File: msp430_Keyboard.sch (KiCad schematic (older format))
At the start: 16 parts, among them J1 Conn_01x04_Male, SW14 L_Super, SW4 L_Ctrl, SW48 R_Ctrl, SW5 L_Shift, SW53 R_Shift, SW57 Alt_GR, SW60 R_Super, SW61 FUNC, SW9 L_Alt, U1 MSP430F5510IRGZ, Y1 12MHz, Y2 32.768kHz

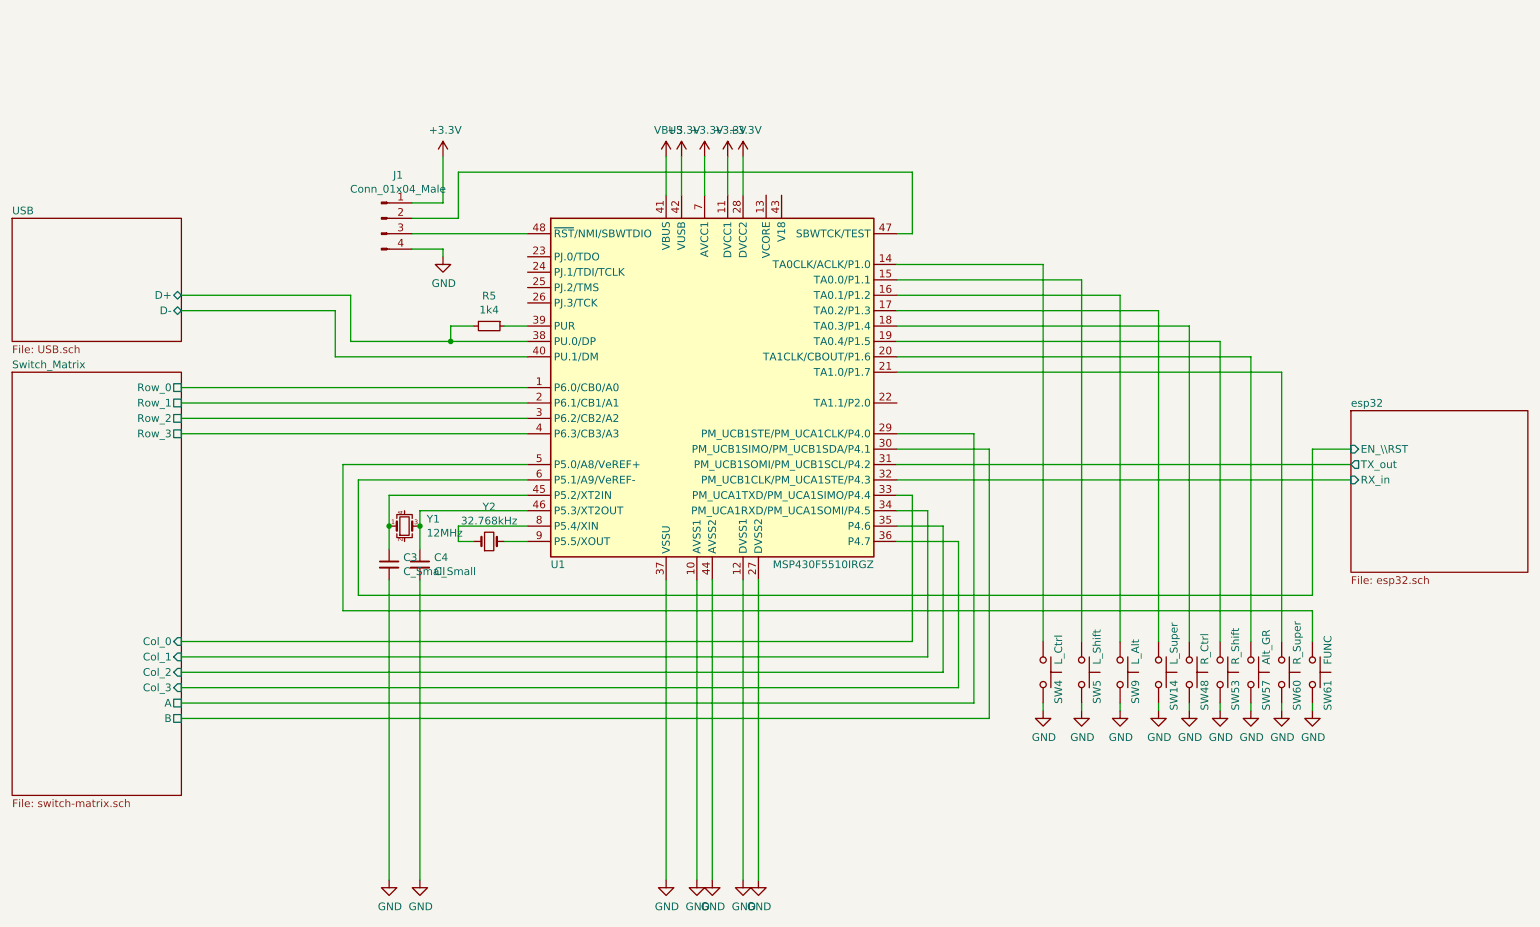
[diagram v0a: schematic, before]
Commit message: Routing angefangen
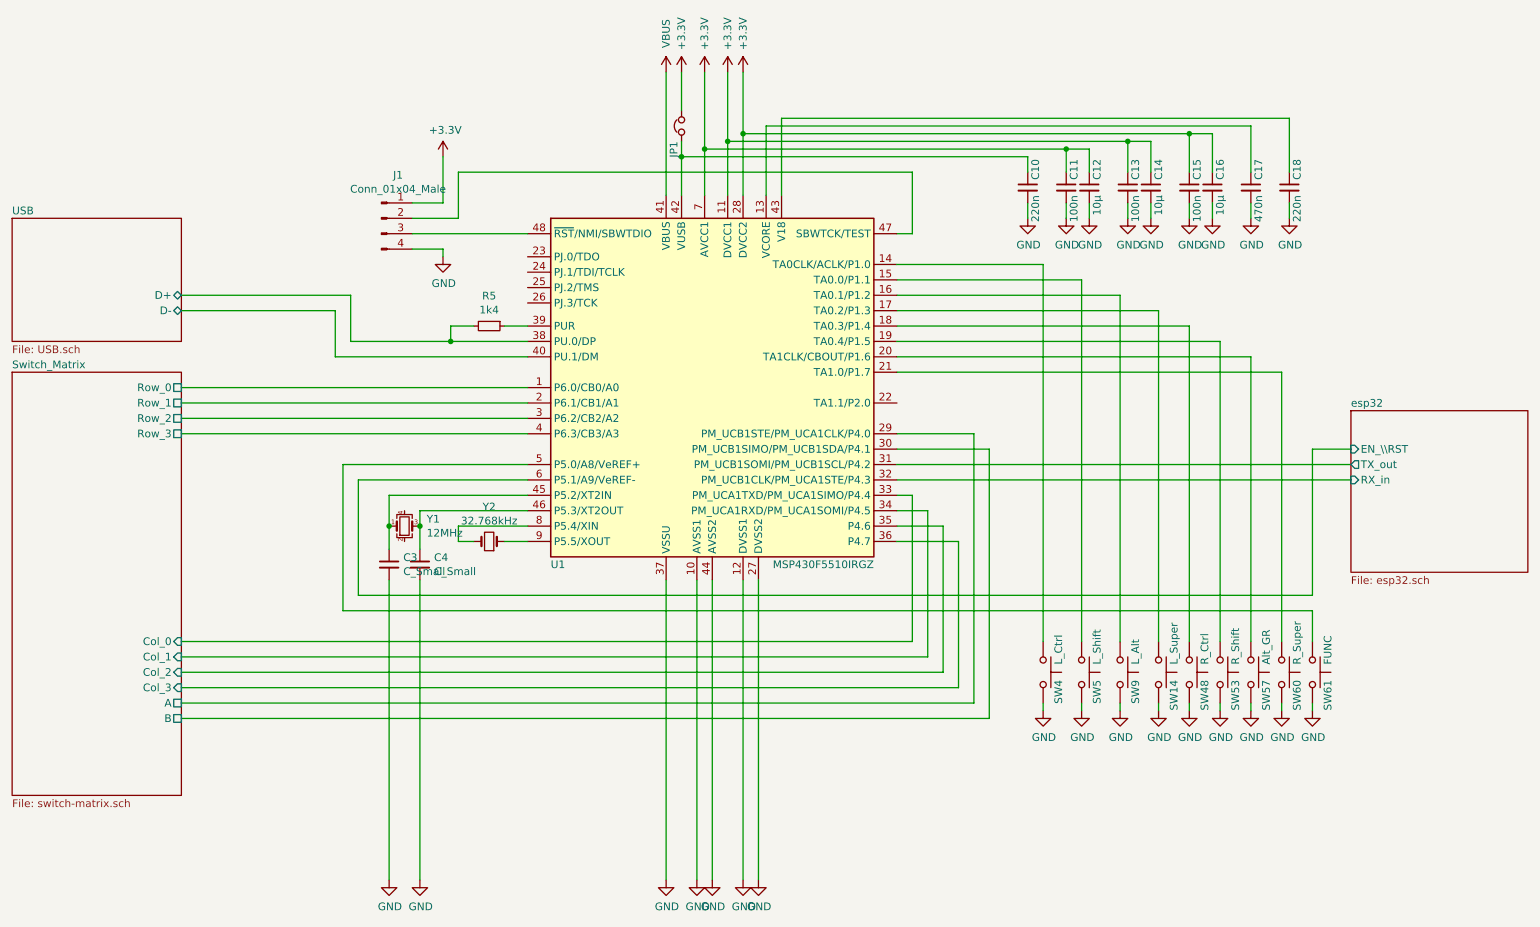
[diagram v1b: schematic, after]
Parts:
- added C10, C18: 220n, Capacitor_SMD:C_0603_1608Metric_Pad1.08x0.95mm_HandSolder, symbol Device:C_Small
- added C11, C13, C15: 100n, Capacitor_SMD:C_0603_1608Metric_Pad1.08x0.95mm_HandSolder, symbol Device:C_Small
- added C12, C14, C16: 10µ, Capacitor_SMD:C_1206_3216Metric_Pad1.33x1.80mm_HandSolder, symbol Device:C_Small
- added C17: 470n, Capacitor_SMD:C_0603_1608Metric_Pad1.08x0.95mm_HandSolder, symbol Device:C_Small
- added JP1: Jumper_NC_Small, Jumper:SolderJumper-2_P1.3mm_Bridged2Bar_RoundedPad1.0x1.5mm, symbol Device:Jumper_NC_Small
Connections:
- net +3V3: now also C11.1, C12.1, C13.1, C14.1, C15.1, C16.1, JP1.2; no longer U1.42 (VUSB)
- net GND: now also C10.2, C11.2, C12.2, C13.2, C14.2, C15.2, C16.2, C17.2, C18.2
- net at U1.13 (VCORE): now also C17.1
- net at U1.43 (V18): now also C18.1
- net at U1.8 (P5.4/XIN): now also Y2.2; no longer Y2.1
- net at U1.9 (P5.5/XOUT): now also Y2.1; no longer Y2.2
- new net: C10.1, JP1.1, U1.42 (VUSB)
